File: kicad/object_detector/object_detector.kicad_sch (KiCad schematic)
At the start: 16 parts, among them U1 LM386

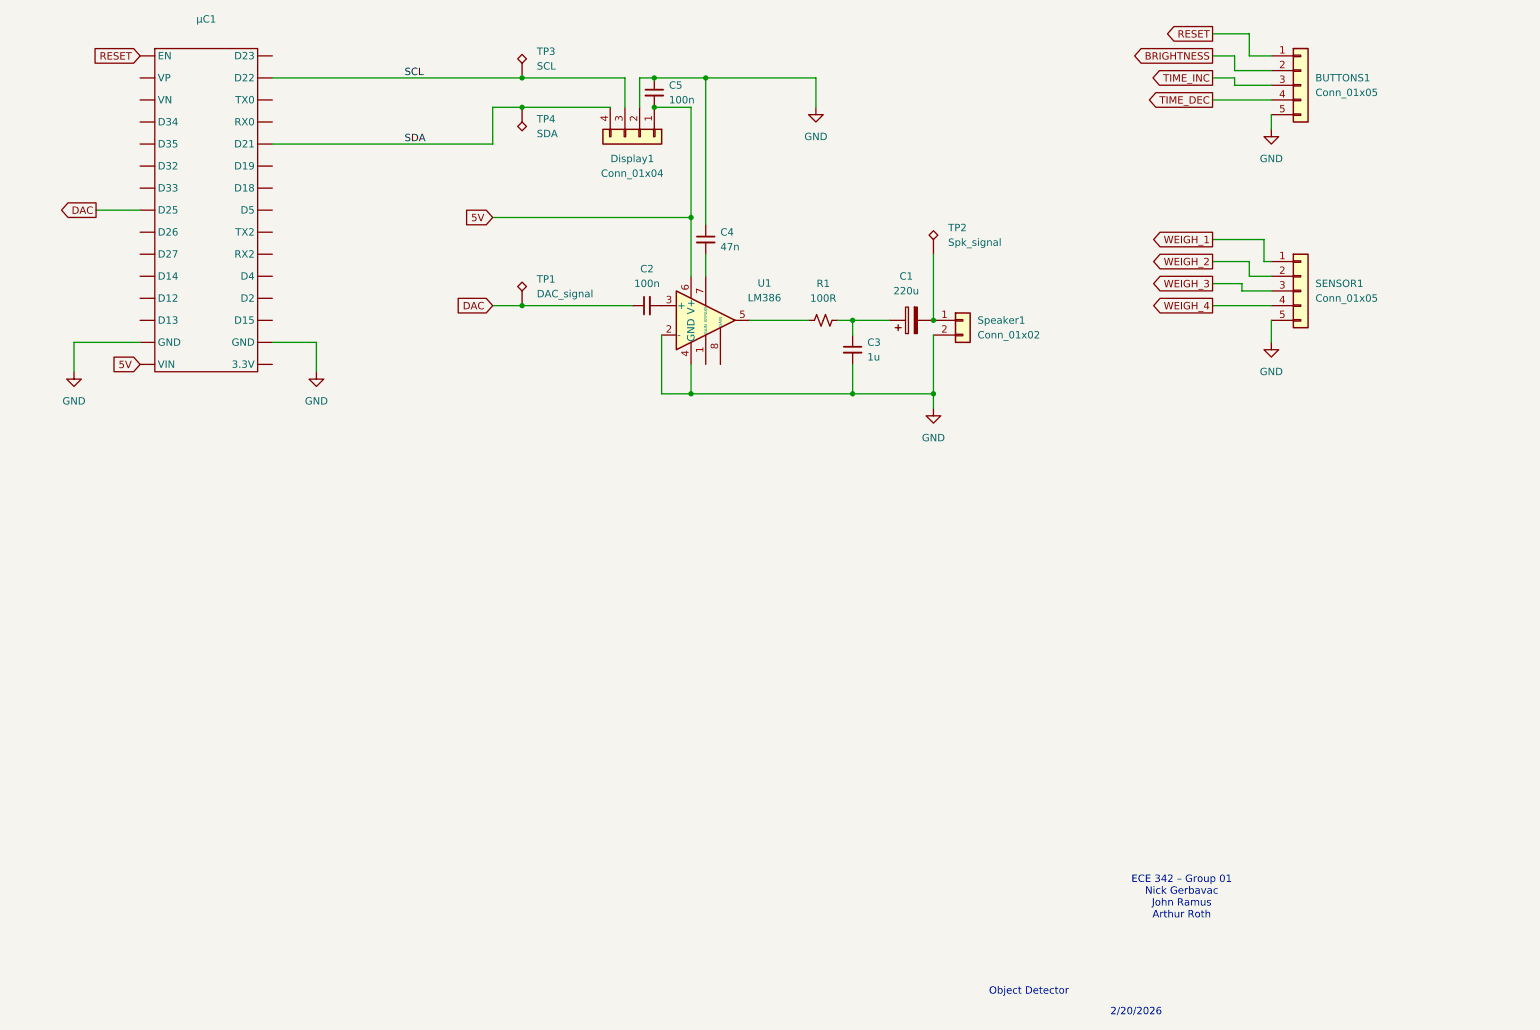
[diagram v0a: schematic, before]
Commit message: updated PCB schematic
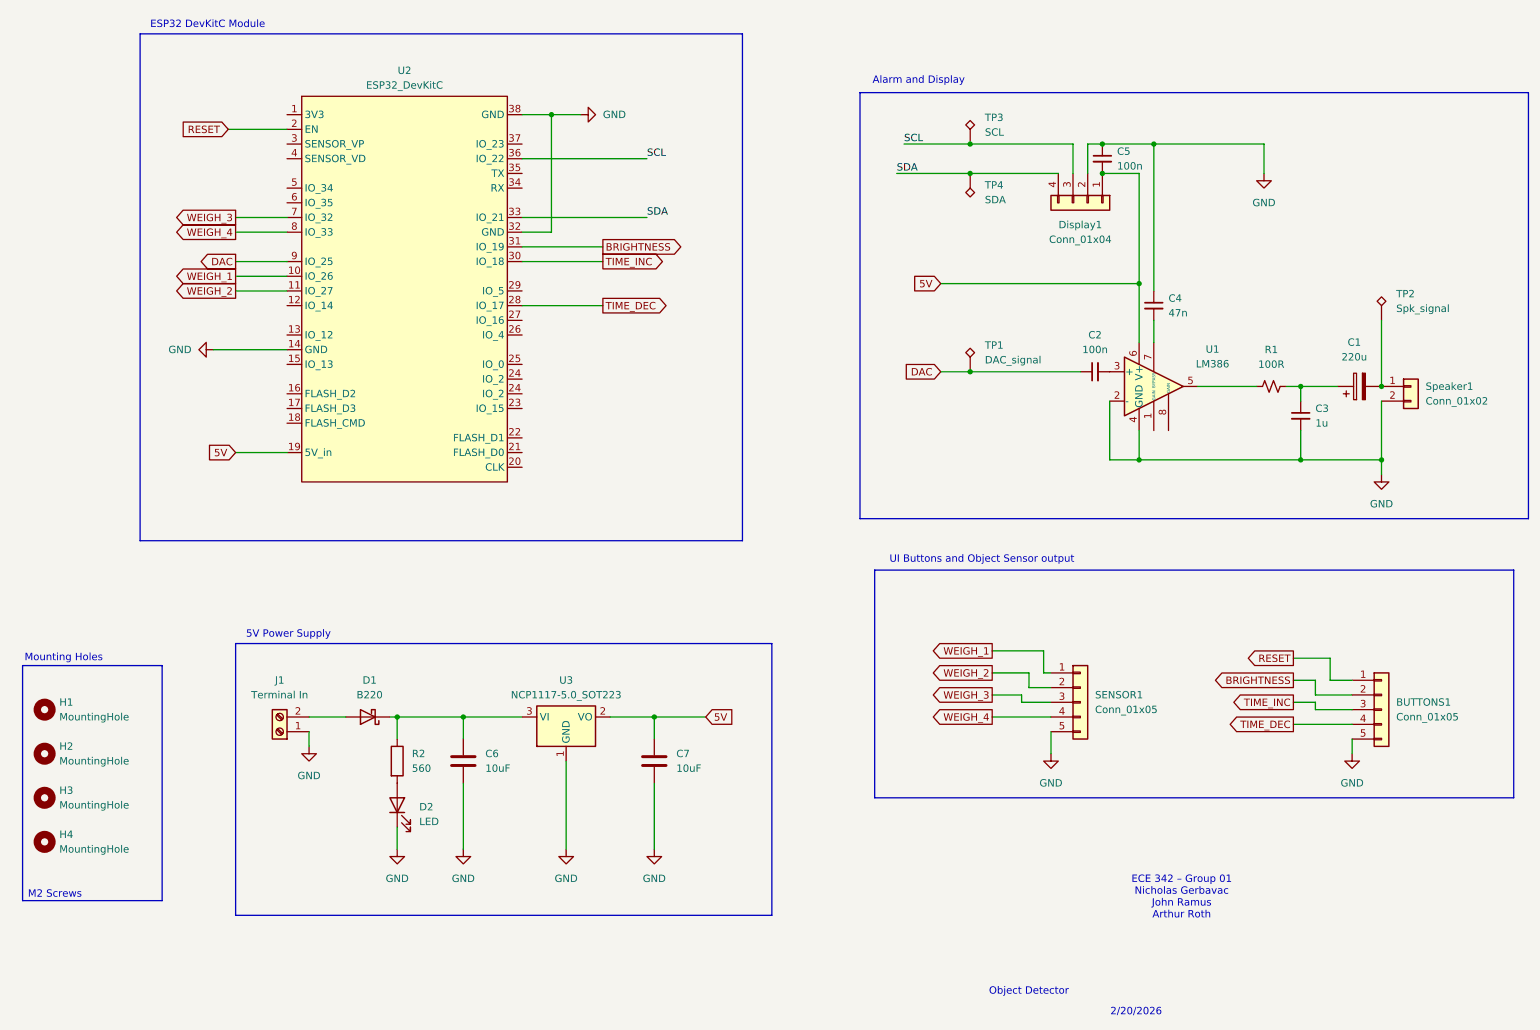
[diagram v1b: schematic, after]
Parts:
- removed µC1: ~, RF_Module:ESP32-C3-DevKitM-1, symbol custom_ece342:ESP32_WROOM
- added C6, C7: 10uF, Capacitor_SMD:C_1206_3216Metric, symbol Device:C
- added D1: B220, Diode_SMD:D_SMA, symbol Device:D_Schottky
- added D2: LED, LED_SMD:LED_0603_1608Metric, symbol Device:LED
- added H1, H2, H3, H4: MountingHole, MountingHole:MountingHole_2.2mm_M2, symbol Mechanical:MountingHole
- added J1: Terminal In, TerminalBlock_TE-Connectivity:TerminalBlock_TE_282834-2_1x02_P2.54mm_Horizontal, symbol Connector:Screw_Terminal_01x02
- added R2: 560, Resistor_SMD:R_0805_2012Metric, symbol Device:R
- added U2: ESP32_DevKitC, ESP32:ESP32_DevKitC_38pin_socket, symbol ESP32:ESP32_DevKitC
- added U3: NCP1117-5.0_SOT223, Package_TO_SOT_SMD:SOT-223-3_TabPin2, symbol ncp1117-5.0_sot223:NCP1117-5.0_SOT223
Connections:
- net 5V: now also C7.1, U2.19 (5V_in), U3.2 (VO)
- net BRIGHTNESS: now also U2.31 (IO_19)
- net DAC: now also U2.9 (IO_25)
- net GND: now also C6.2, C7.2, D2.1 (K), J1.1 (Pin_1), U2.14 (GND), U2.32 (GND), U2.38 (GND), U3.1 (GND)
- net RESET: now also U2.2 (EN)
- net SCL: now also U2.36 (IO_22)
- net SDA: now also U2.33 (IO_21)
- net TIME_DEC: now also U2.28 (IO_17)
- net TIME_INC: now also U2.30 (IO_18)
- net WEIGH_1: now also U2.10 (IO_26)
- net WEIGH_2: now also U2.11 (IO_27)
- net WEIGH_3: now also U2.7 (IO_32)
- net WEIGH_4: now also U2.8 (IO_33)
- new net: C6.1, D1.1 (K), R2.1, U3.3 (VI)
- new net: D2.2 (A), R2.2
- new net: D1.2 (A), J1.2 (Pin_2)
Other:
- note added: "5V Power Supply"
- note added: "Alarm and Display"
- note added: "ECE 342 – Group 01 Nicholas Gerbavac John Ramus Arthur Roth"
- note added: "ESP32 DevKitC Module"
- note added: "M2 Screws"
- note added: "Mounting Holes"
- note added: "UI Buttons and Object Sensor output"
- note removed: "ECE 342 – Group 01 Nick Gerbavac John Ramus Arthur Roth"
- moved on the sheet: BUTTONS1, C1, C2, C3, C4, C5, Display1, R1, SENSOR1, Speaker1, TP1, TP2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
